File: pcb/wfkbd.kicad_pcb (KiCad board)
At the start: 2 copper layers, 114 parts, among them J1 MJ-4PP-9, P1 LED, SW1 KEY, SW10 KEY, SW11 KEY, SW12 KEY, SW13 KEY, SW14 KEY, SW15 KEY, SW16 KEY, SW17 KEY, SW18 KEY, SW19 KEY, SW2 KEY, SW20 KEY, SW21 KEY, SW22 KEY, SW23 KEY, SW24 KEY, SW25 KEY, SW26 KEY, SW27 KEY, SW28 KEY, SW29 KEY, SW3 KEY, SW30 KEY, SW31 KEY, SW32 KEY, SW33 KEY, SW34 KEY, SW35 KEY, SW4 KEY, SW5 KEY, SW6 KEY, SW7 KEY, SW8 KEY, SW9 KEY, U1 ProMicro

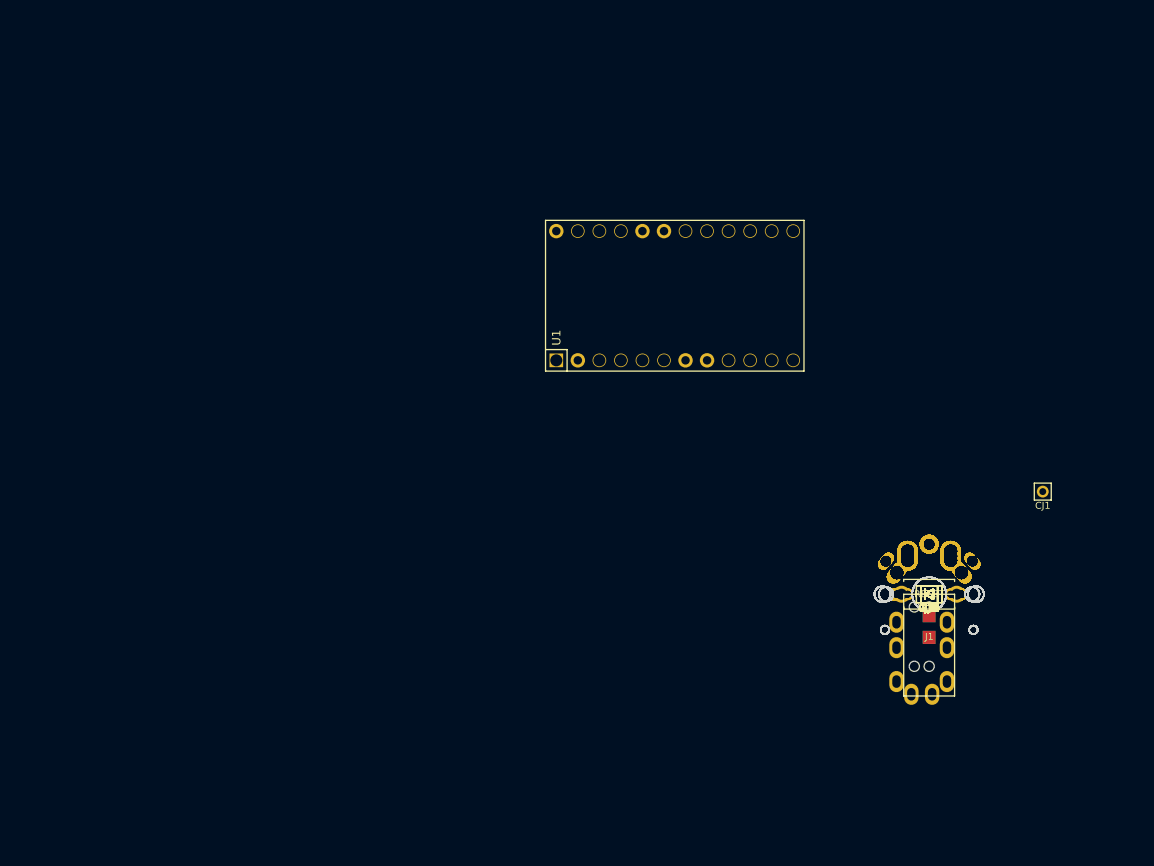
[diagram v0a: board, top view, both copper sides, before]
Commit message: Add pcbnew files
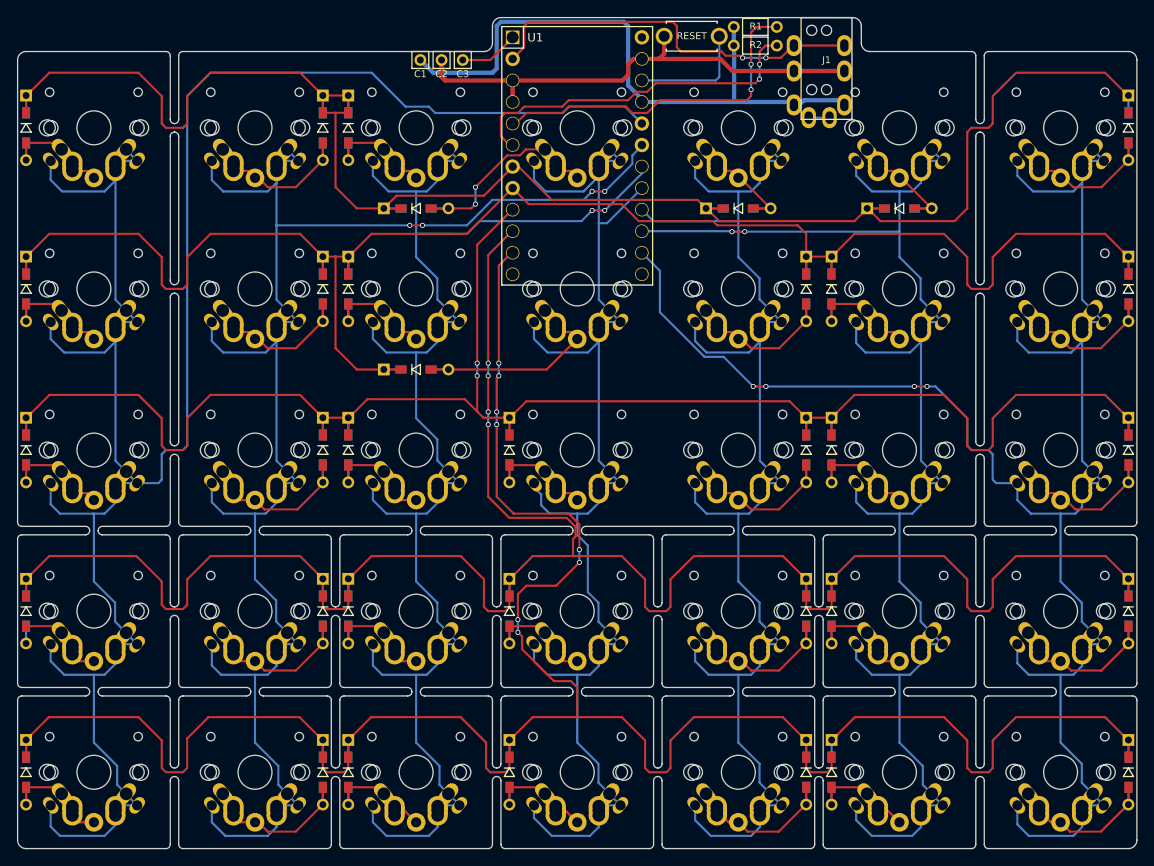
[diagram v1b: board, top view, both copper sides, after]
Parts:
- removed CJ1, CJ15, CJ22, CJ8: col0, kbd:1pin_conn
- removed CJ10, CJ17, CJ24, CJ3: col2, kbd:1pin_conn
- removed CJ11, CJ18, CJ25, CJ4: col3, kbd:1pin_conn
- removed CJ12, CJ19, CJ26, CJ5: col4, kbd:1pin_conn
- removed CJ13, CJ20, CJ27, CJ6: col5, kbd:1pin_conn
- removed CJ14, CJ21, CJ28, CJ7: col6, kbd:1pin_conn
- removed CJ16, CJ2, CJ23, CJ9: col1, kbd:1pin_conn
- removed P1: LED, kbd:StripLED_rev
- removed RJ1, RJ10, RJ2, RJ3, RJ4, RJ5, RJ6, RJ7, RJ8, RJ9: row0, kbd:1pin_conn
- added C1: VCC, kbd:1pin_conn, F.Cu at (88.5, 42.0)
- added C2: GND, kbd:1pin_conn, F.Cu at (91.0, 42.0)
- added C3: LED, kbd:1pin_conn, F.Cu at (93.5, 42.0)
- moved D1 119.9 mm to (42.0, 50.0), turned to 270 degrees
- moved SW1 112.8 mm to (50.0, 50.0), turned to 180 degrees
- moved D8 112.4 mm to (42.0, 69.0), turned to 270 degrees
- moved D29 108.6 mm to (42.0, 126.0), turned to 270 degrees
- moved D15 107.8 mm to (42.0, 88.0), turned to 270 degrees
- moved D22 106.5 mm to (42.0, 107.0), turned to 270 degrees
- moved SW8 104.9 mm to (50.0, 69.0), turned to 180 degrees
- moved SW29 100.7 mm to (50.0, 126.0), turned to 180 degrees
- moved SW15 100.0 mm to (50.0, 88.0), turned to 180 degrees
- moved SW22 98.5 mm to (50.0, 107.0), turned to 180 degrees
- moved SW2 96.7 mm to (69.0, 50.0), turned to 180 degrees
- moved D2 90.2 mm to (77.0, 50.0), turned to 270 degrees
- moved D3 87.9 mm to (80.0, 50.0), turned to 270 degrees
- moved SW9 87.3 mm to (69.0, 69.0), turned to 180 degrees
- moved SW30 82.2 mm to (69.0, 126.0), turned to 180 degrees
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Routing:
- net row4: track 0.00 -> 276.4 mm, vias 0 -> 8
- net col0: track 0.00 -> 262.2 mm
- net row3: track 0.00 -> 254.8 mm, vias 0 -> 4
- net col6: track 0.00 -> 216.0 mm, vias 0 -> 4
- net row2: track 0.00 -> 210.4 mm, vias 0 -> 2
- net row1: track 0.00 -> 207.2 mm
- net row0: track 0.00 -> 203.8 mm
- net col1: track 0.00 -> 200.4 mm, vias 0 -> 4
- net col5: track 0.00 -> 182.4 mm, vias 0 -> 2
- net col2: track 0.00 -> 180.9 mm, vias 0 -> 2
- net col4: track 0.00 -> 164.1 mm
- net col3: track 0.00 -> 159.4 mm
- net VCC: track 0.00 -> 73.7 mm
- net GND: track 0.00 -> 57.6 mm
- net data: track 0.00 -> 46.6 mm, vias 0 -> 2
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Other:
- board outline added: 132 x 98 mm
